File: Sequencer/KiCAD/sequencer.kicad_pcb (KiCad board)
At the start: 2 copper layers, 73 x 27 mm, 22 parts, among them J1 12V -13,8V DC, J2 MCU 11, J3 GX12, Q1 BC237, Q2 BC237, Q3 PNP

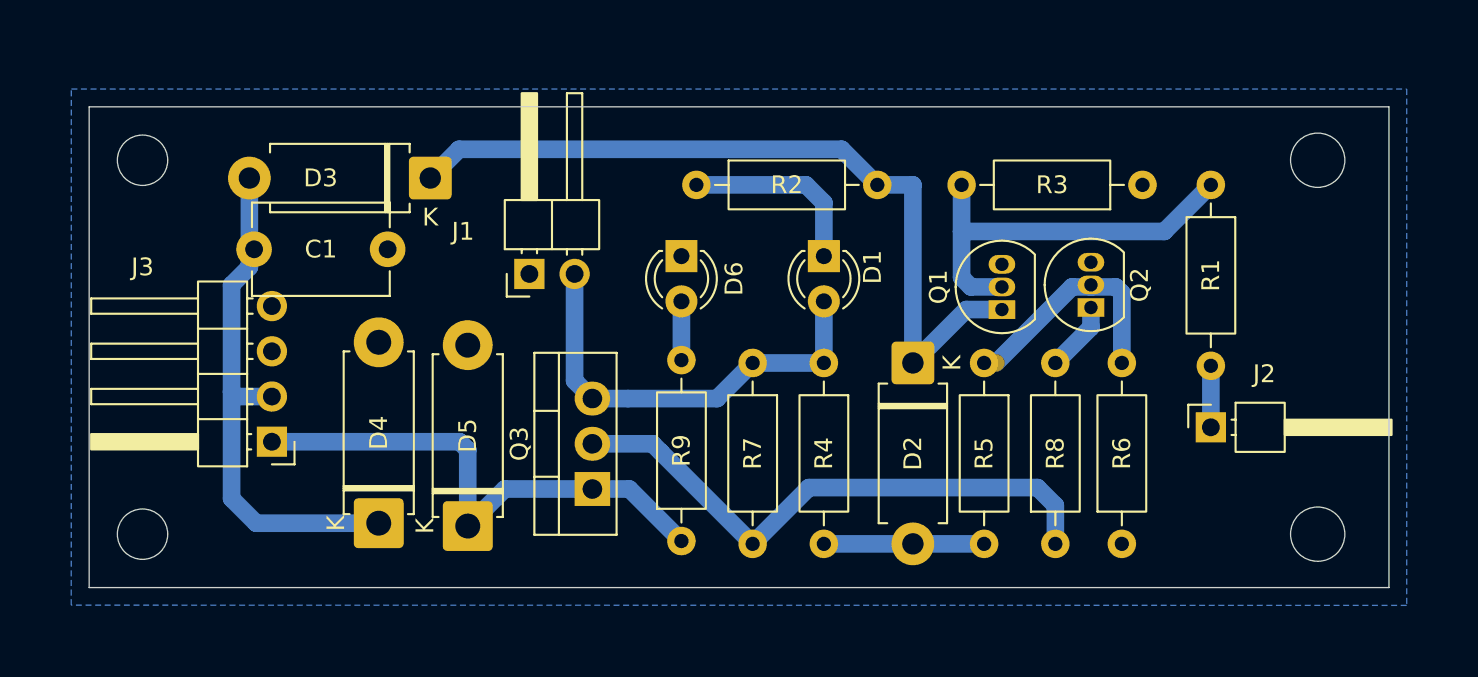
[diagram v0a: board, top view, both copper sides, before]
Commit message: 3.7.26
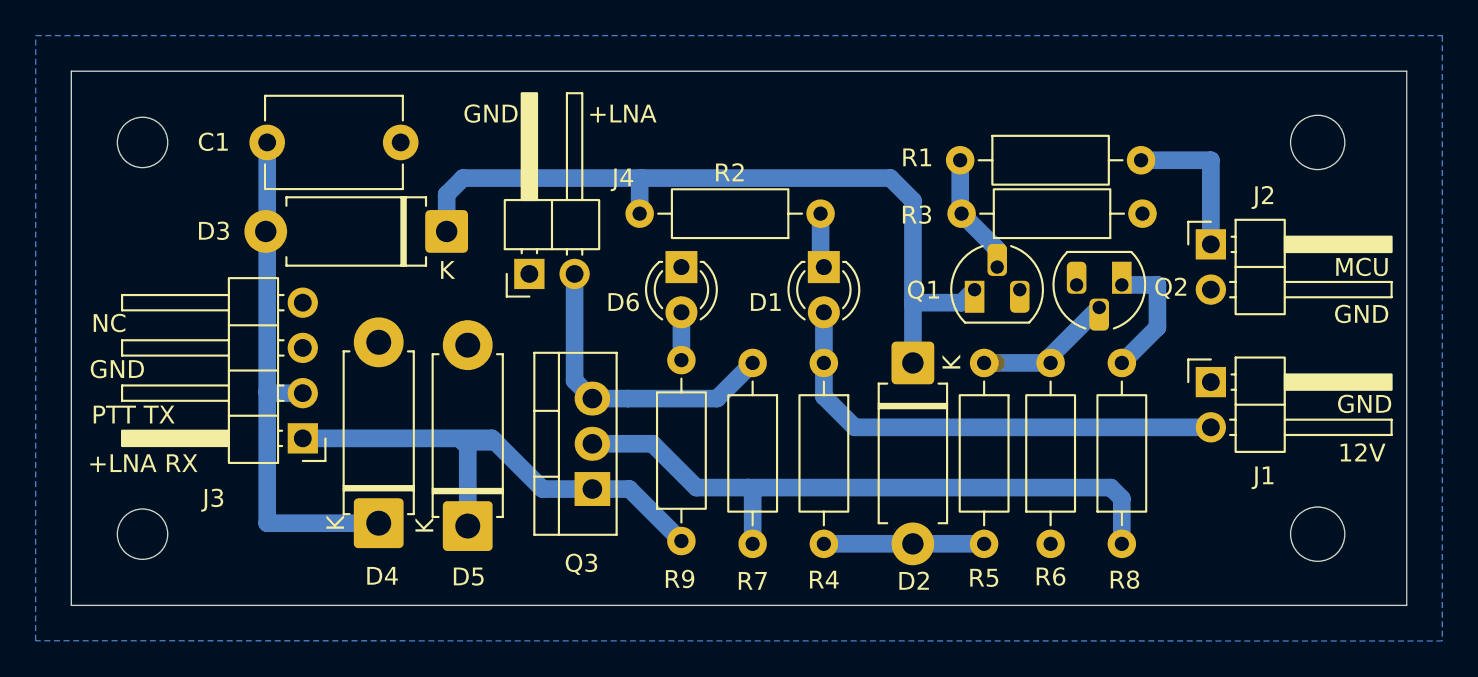
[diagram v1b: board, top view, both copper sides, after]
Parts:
- added J4: 12V, Connector_PinHeader_2.54mm:PinHeader_1x02_P2.54mm_Horizontal, F.Cu at (128.7, 92.4)
- J1: value 12V -13,8V DC -> 12V DC
- J2: value MCU 11 -> MCU; footprint Connector_PinHeader_2.54mm:PinHeader_1x01_P2.54mm_Horizontal -> Connector_PinHeader_2.54mm:PinHeader_1x02_P2.54mm_Horizontal
- Q1, Q2: footprint Package_TO_SOT_THT:TO-92_Inline -> Package_TO_SOT_THT:TO-92L_HandSolder
- moved J1 38.8 mm to (167.0, 98.5), turned to 0 degrees
- moved R1 14.1 mm to (152.9, 86.0), turned to 0 degrees
- moved J2 10.3 mm to (167.0, 90.7)
- moved R2 7.16 mm to (145.1, 89.0), turned to 180 degrees
- moved C1 6.04 mm to (114.0, 85.0)
- moved R6 4.00 mm to (158.0, 107.5)
- moved R8 3.74 mm to (162.0, 107.5)
- moved D3 3.14 mm to (124.1, 90.0)
- moved Q2 2.15 mm to (162.0, 93.0), turned to 180 degrees
- moved Q1 1.90 mm to (153.7, 93.3), turned to 0 degrees
- moved J3 1.75 mm to (116.0, 101.6)
- moved R3 1.61 mm to (163.2, 89.0)
- moved D1 0.61 mm to (145.3, 92.0)
- moved D6 0.61 mm to (137.3, 92.0)
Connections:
- D1 pad 2: +VIN -> +12V
- J1 pad 2: +VIN -> +12V
- Q3 pad 3: +VIN -> +LNA
- R4 pad 1: +VIN -> +12V
- R7 pad 1: +VIN -> +LNA
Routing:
- net +12V: track 0.00 -> 27.2 mm
- net +VIN: track 24.7 -> 0.00 mm
- net +LNA: track 0.00 -> 17.2 mm
- net Net-(Q1-B): track 22.8 -> 6.86 mm
- net Net-(D1-K): track 10.6 -> 3.34 mm
- net Net-(J2-Pin_1): track 3.45 -> 8.64 mm
- net Net-(Q2-B): track 13.6 -> 8.65 mm
- net Net-(Q3-B): track 32.2 -> 36.8 mm
- net Net-(Q2-C): track 3.83 -> 7.21 mm
- net Net-(D5-K): track 29.5 -> 30.3 mm
- net Net-(D2-K): track 44.8 -> 44.1 mm
- net Net-(D6-A): track 3.30 -> 2.68 mm
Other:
- board size 73 x 27 mm -> 75 x 30 mm
- board text added: "+LNA"
- board text added: "+LNA RX"
- board text added: "12V"
- board text added: "GND"
- board text added: "MCU"
- board text added: "NC"
- board text added: "PTT TX"
